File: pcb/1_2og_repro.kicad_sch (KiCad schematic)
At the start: 222 parts, among them J1 Pico EzMate, J2 USB_B_Mini, J3 Raw Header, J4 JST PH S3B, J5 Foam, SW1 MX_SW_solder, SW10 MX_SW_solder, SW11 MX_SW_solder, SW12 MX_SW_solder, SW13 MX_SW_solder, SW14 MX_SW_solder, SW15 MX_SW_solder, SW16 MX_SW_solder, SW17 MX_SW_solder, SW18 MX_SW_solder, SW19 MX_SW_solder, SW2 MX_SW_solder, SW20 MX_SW_solder, SW21 MX_SW_solder, SW22 MX_SW_solder, SW23 MX_SW_solder, SW24 MX_SW_solder, SW25 MX_SW_solder, SW26 MX_SW_solder, SW27 MX_SW_solder, SW28 MX_SW_solder, SW29 MX_SW_solder, SW3 MX_SW_solder, SW30 MX_SW_solder, SW31 MX_SW_solder, SW32 MX_SW_solder, SW33 MX_SW_solder, SW34 MX_SW_solder, SW35 MX_SW_solder, SW36 MX_SW_solder, SW37 MX_SW_solder, SW38 MX_SW_solder, SW39 MX_SW_solder, SW4 MX_SW_solder, SW40 MX_SW_solder, SW41 MX_SW_solder, SW42 MX_SW_solder, SW43 MX_SW_solder, SW44 MX_SW_solder, SW45 MX_SW_solder, SW46 MX_SW_solder, SW47 MX_SW_solder, SW48 MX_SW_solder, SW49 MX_SW_solder, SW5 MX_SW_solder, SW50 MX_SW_solder, SW51 MX_SW_solder, SW52 MX_SW_solder, SW53 MX_SW_solder, SW54 MX_SW_solder, SW55 MX_SW_solder, SW56 MX_SW_solder, SW57 MX_SW_solder, SW58 MX_SW_solder, SW59 MX_SW_solder, SW6 MX_SW_solder, SW60 MX_SW_solder, SW61 MX_SW_solder, SW62 MX_SW_solder, SW63 MX_SW_solder, SW64 MX_SW_solder, SW65 MX_SW_solder, SW66 MX_SW_solder, SW67 MX_SW_solder, SW68 MX_SW_solder, SW69 MX_SW_solder, SW7 MX_SW_solder, SW70 MX_SW_solder, SW71 MX_SW_solder, SW72 MX_SW_solder, SW73 MX_SW_solder, SW74 MX_SW_solder, SW75 MX_SW_solder, SW76 MX_SW_solder, SW77 MX_SW_solder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

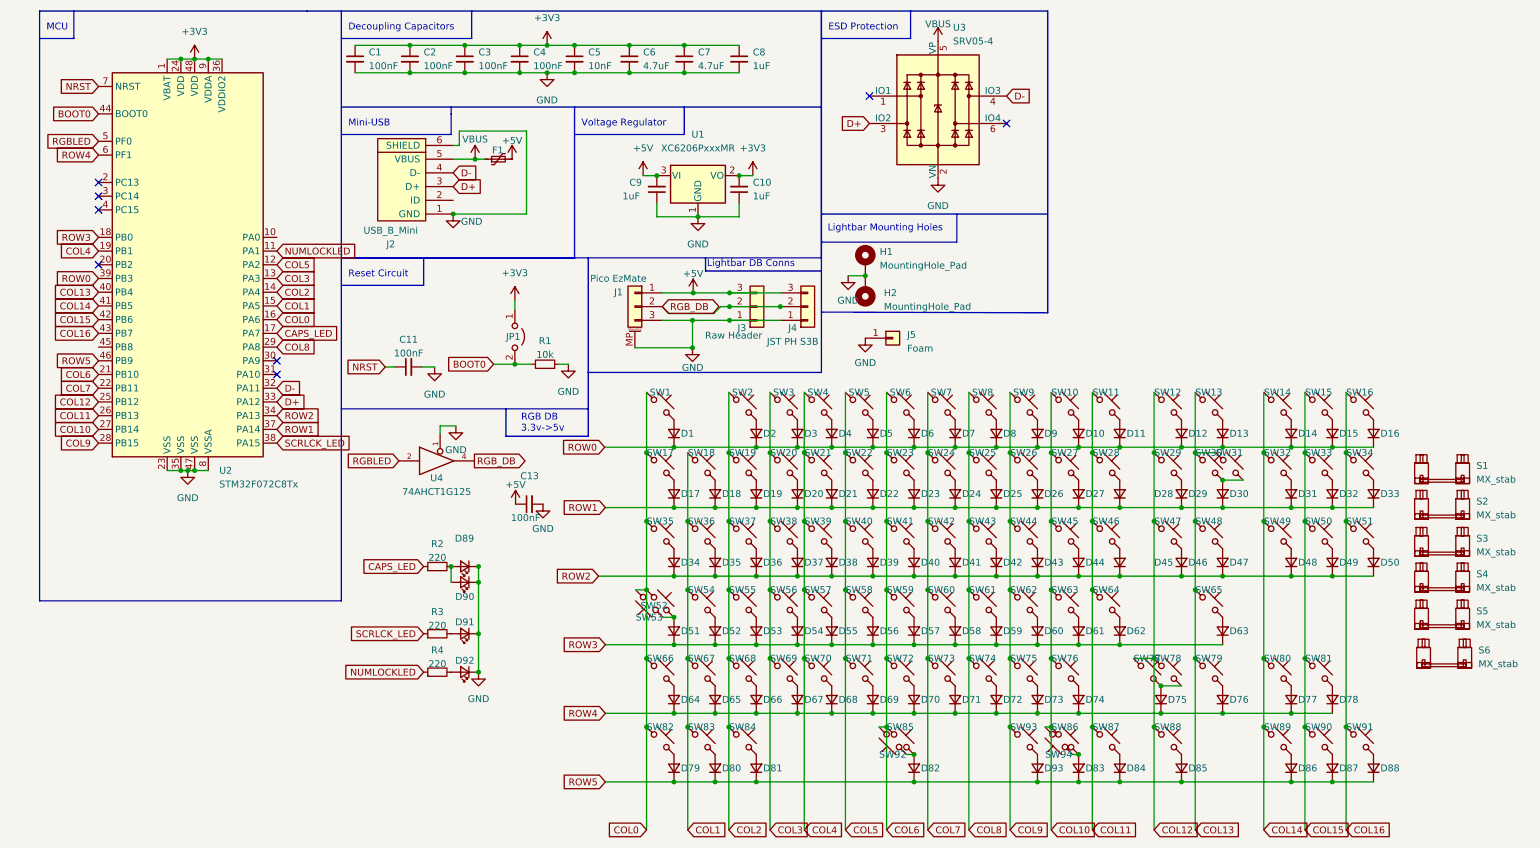
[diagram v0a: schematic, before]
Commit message: REMAKE - FIRMWARE NEEDS UPDATES
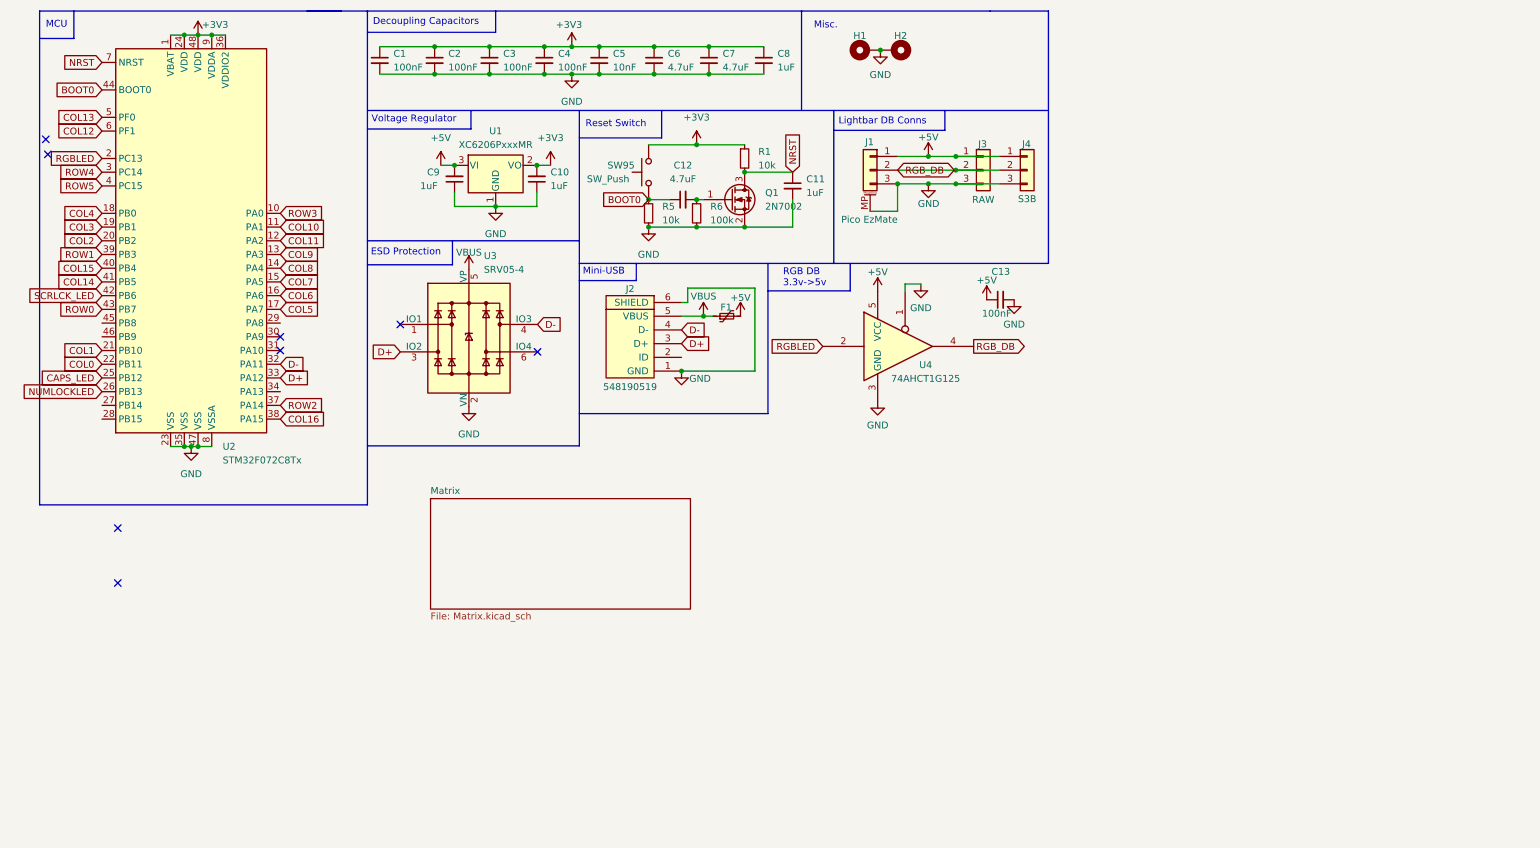
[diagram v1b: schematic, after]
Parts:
- removed D1, D10, D11, D12, D13, D14, D15, D16, D17, D18, D19, D2, D20, D21, D22, D23, D24, D25, D26, D27, D28, D29, D3, D30, D31, D32, D33, D34, D35, D36, D37, D38, D39, D4, D40, D41, D42, D43, D44, D45, D46, D47, D48, D49, D5, D50, D51, D52, D53, D54, D55, D56, D57, D58, D59, D6, D60, D61, D62, D63, D64, D65, D66, D67, D68, D69, D7, D70, D71, D72, D73, D74, D75, D76, D77, D78, D79, D8, D80, D81, D82, D83, D84, D85, D86, D87, D88, D9, D93: D_Small, Diode_SMD:D_SOD-123, symbol Device:D_Small
- removed D89, D91, D92: LED_Small, marbastlib-mx:LED_MX_3mm, symbol Device:LED_Small
- removed D90: LED_Small, marbastlib-mx:LED_MX_3mm-ROT, symbol Device:LED_Small
- removed J5: Foam, Connector_Wire:SolderWirePad_1x01_SMD_5x10mm, symbol Connector_Generic:Conn_01x01
- removed JP1: Jumper_2_Open, TestPoint:TestPoint_2Pads_Pitch5.08mm_Drill1.3mm, symbol Jumper:Jumper_2_Open
- removed R2, R3, R4: 220, Resistor_SMD:R_0402_1005Metric, symbol Device:R_Small
- removed S1: MX_stab, marbastlib-mx:STAB_MX_P_2u, symbol marbastlib-mx:MX_stab
- removed S2, S3: MX_stab, marbastlib-mx:STAB_MX_2.25u, symbol marbastlib-mx:MX_stab
- removed S4: MX_stab, marbastlib-mx:STAB_MX_P_2.75u, symbol marbastlib-mx:MX_stab
- removed S5: MX_stab, marbastlib-mx:STAB_MX_7u, symbol marbastlib-mx:MX_stab
- removed S6: MX_stab, marbastlib-mx:STAB_MX_6u, symbol marbastlib-mx:MX_stab
- removed SW1, SW10, SW11, SW12, SW13, SW14, SW15, SW16, SW17, SW18, SW19, SW2, SW20, SW21, SW22, SW23, SW24, SW25, SW26, SW27, SW28, SW29, SW3, SW30, SW31, SW32, SW33, SW34, SW36, SW37, SW38, SW39, SW4, SW40, SW41, SW42, SW43, SW44, SW45, SW46, SW47, SW49, SW5, SW50, SW51, SW54, SW55, SW56, SW57, SW58, SW59, SW6, SW60, SW61, SW62, SW63, SW64, SW65, SW66, SW67, SW68, SW69, SW7, SW70, SW71, SW72, SW73, SW74, SW75, SW76, SW78, SW79, SW8, SW80, SW81, SW83, SW85, SW87, SW89, SW9, SW90, SW91, SW92, SW94: MX_SW_solder, marbastlib-mx:SW_MX_1u, symbol marbastlib-mx:MX_SW_solder
- removed SW35, SW48, SW82, SW84, SW86, SW88, SW93: MX_SW_solder, marbastlib-mx:SW_MX_1.5u, symbol marbastlib-mx:MX_SW_solder
- removed SW52: MX_SW_solder, marbastlib-mx:SW_MX_1.75u_STP_1.25, symbol marbastlib-mx:MX_SW_solder
- removed SW53, SW77: MX_SW_solder, marbastlib-mx:SW_MX_1.75u, symbol marbastlib-mx:MX_SW_solder
- added C12: 4.7uF, Capacitor_SMD:C_0402_1005Metric, symbol Device:C_Small
- added Q1: 2N7002, Package_TO_SOT_SMD:SOT-23, symbol Transistor_FET:2N7002
- added R5: 10k, Resistor_SMD:R_0402_1005Metric, symbol Device:R_Small
- added R6: 100k, Resistor_SMD:R_0402_1005Metric, symbol Device:R_Small
- added SW95: SW_Push, Button_Switch_SMD:SW_SPST_TL3342, symbol Switch:SW_Push
- C11: value 100nF -> 1uF
- J2: value USB_B_Mini -> 548190519; footprint random-keyboard-parts:Molex-0548190589 -> random-keyboard-parts:Molex-0548190519
- J3: value Raw Header -> RAW
- J4: value JST PH S3B -> S3B
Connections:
- net +3V3: now also R1.1, SW95.2
- net +5V: now also J3.1 (Pin_1), J4.1 (Pin_1); no longer J3.3 (Pin_3), J4.3 (Pin_3)
- net BOOT0: now also C12.1, R5.1, SW95.1; no longer R1.2
- net CAPS_LED: now also U2.25 (PB12); no longer U2.17 (PA7)
- net COL0: now also U2.22 (PB11); no longer U2.16 (PA6)
- net COL1: now also U2.21 (PB10); no longer U2.15 (PA5)
- net COL10: now also U2.11 (PA1); no longer U2.27 (PB14)
- net COL11: now also U2.12 (PA2); no longer U2.26 (PB13)
- net COL12: now also U2.6 (PF1); no longer U2.25 (PB12)
- net COL13: now also U2.5 (PF0); no longer U2.40 (PB4)
- net COL15: now also U2.40 (PB4); no longer U2.42 (PB6)
- net COL16: now also U2.38 (PA15); no longer U2.43 (PB7)
- net COL2: now also U2.20 (PB2); no longer U2.14 (PA4)
- net COL3: now also U2.19 (PB1); no longer U2.13 (PA3)
- net COL4: now also U2.18 (PB0); no longer U2.19 (PB1)
- net COL5: now also U2.17 (PA7); no longer U2.12 (PA2)
- net COL6: now also U2.16 (PA6); no longer U2.21 (PB10)
- net COL7: now also U2.15 (PA5); no longer U2.22 (PB11)
- net COL8: now also U2.14 (PA4); no longer U2.29 (PA8)
- net COL9: now also U2.13 (PA3); no longer U2.28 (PB15)
- net GND: now also J3.3 (Pin_3), J4.3 (Pin_3), Q1.2 (S), R5.2, R6.2; no longer J3.1 (Pin_1), J4.1 (Pin_1), R1.1
- net NRST: now also R1.2, Q1.3 (D)
- net NUMLOCKLED: now also U2.26 (PB13); no longer U2.11 (PA1)
- net RGBLED: now also U2.2 (PC13); no longer U2.5 (PF0)
- net ROW0: now also U2.43 (PB7); no longer U2.39 (PB3)
- net ROW1: now also U2.39 (PB3); no longer U2.37 (PA14)
- net ROW2: now also U2.37 (PA14); no longer U2.34 (PA13)
- net ROW3: now also U2.10 (PA0); no longer U2.18 (PB0)
- net ROW4: now also U2.3 (PC14); no longer U2.6 (PF1)
- net ROW5: now also U2.4 (PC15); no longer U2.46 (PB9)
- net SCRLCK_LED: now also U2.42 (PB6); no longer U2.38 (PA15)
- new net: C12.2, Q1.1 (G), R6.1
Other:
- added sheet Matrix (Matrix.kicad_sch)
- note added: "Misc."
- note added: "Reset Switch"
- note removed: "Lightbar Mounting Holes"
- note removed: "Reset Circuit"
- moved on the sheet: C1, C10, C13, C2, C3, C4, C5, C6, C7, C8, C9, F1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
